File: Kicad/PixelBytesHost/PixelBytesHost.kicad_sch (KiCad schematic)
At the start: 27 parts, among them IC1 2536030320001, J1 TC2030-MCP-NL, Q1 SMMBT5551LT1G, Q2 SMMBT5551LT1G, U1 Pixel Bytes Display, U2 STM32F103CBTx, Y1 CX2520DB12000D0GPSC1

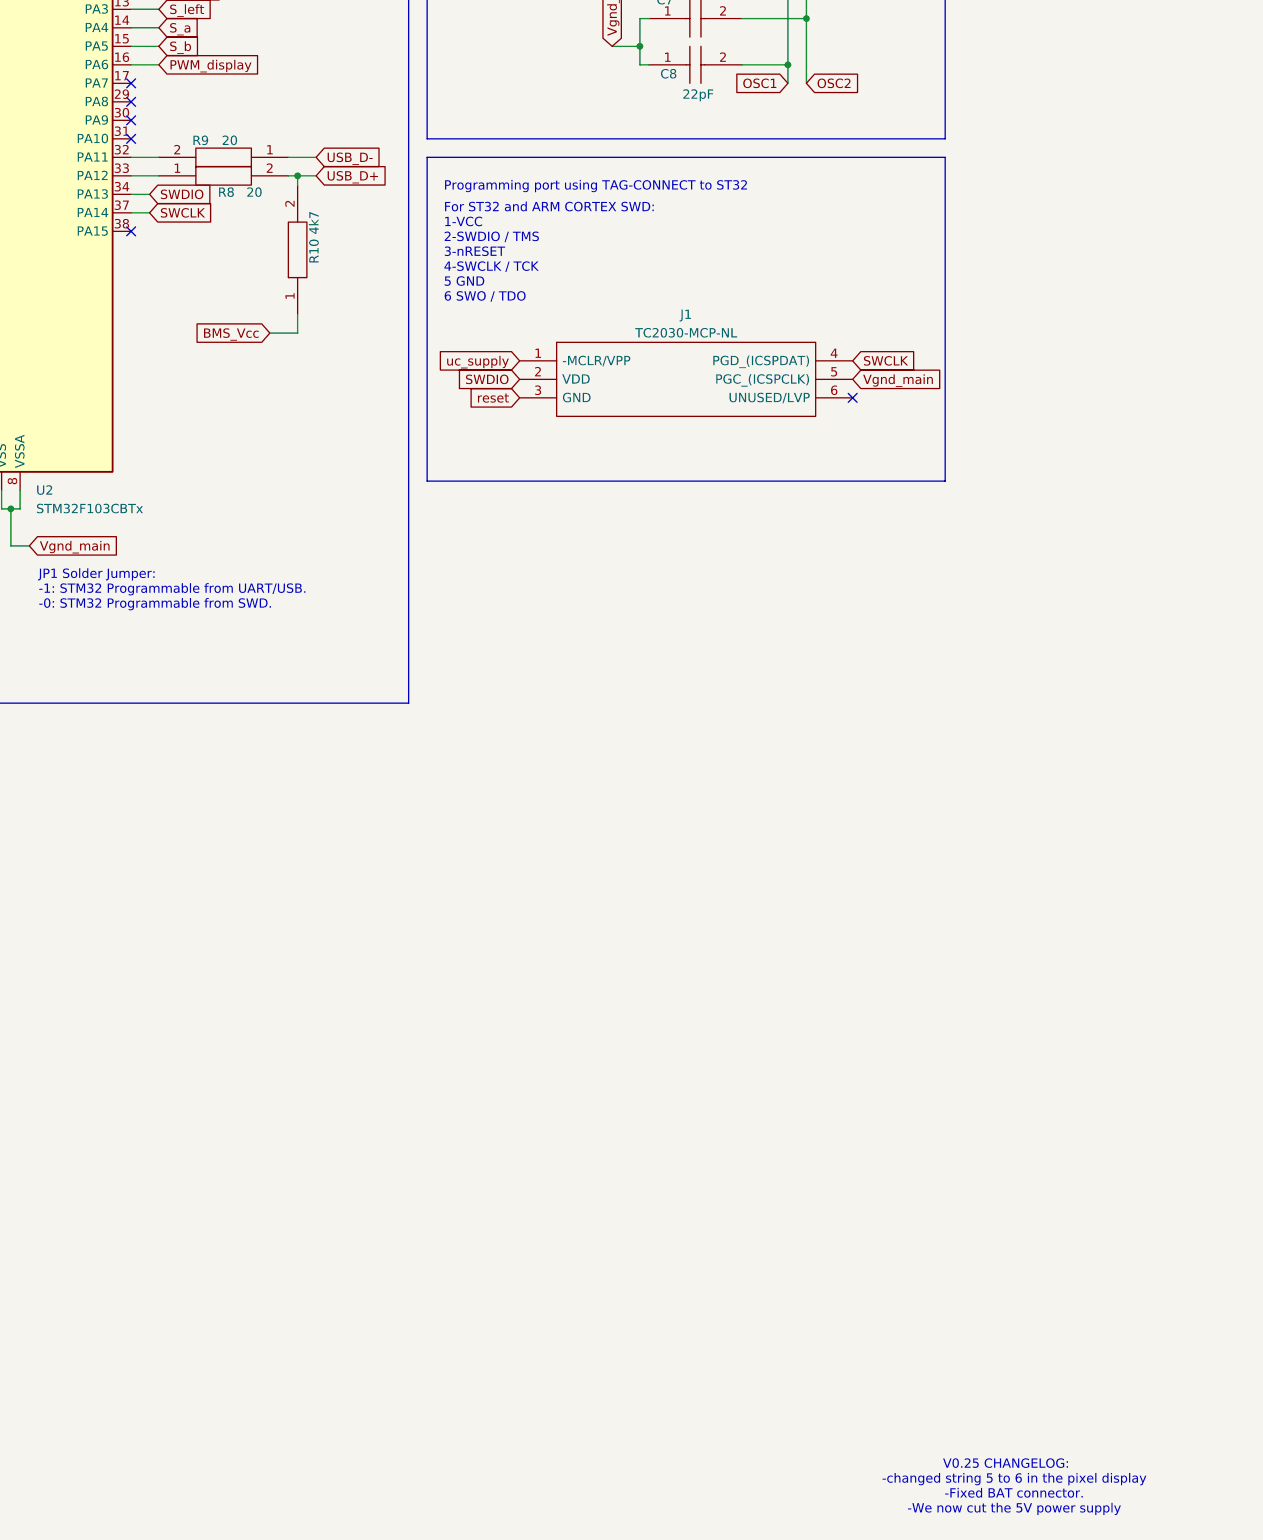
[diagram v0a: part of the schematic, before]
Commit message: Subimos todos los archivos de la v0.25
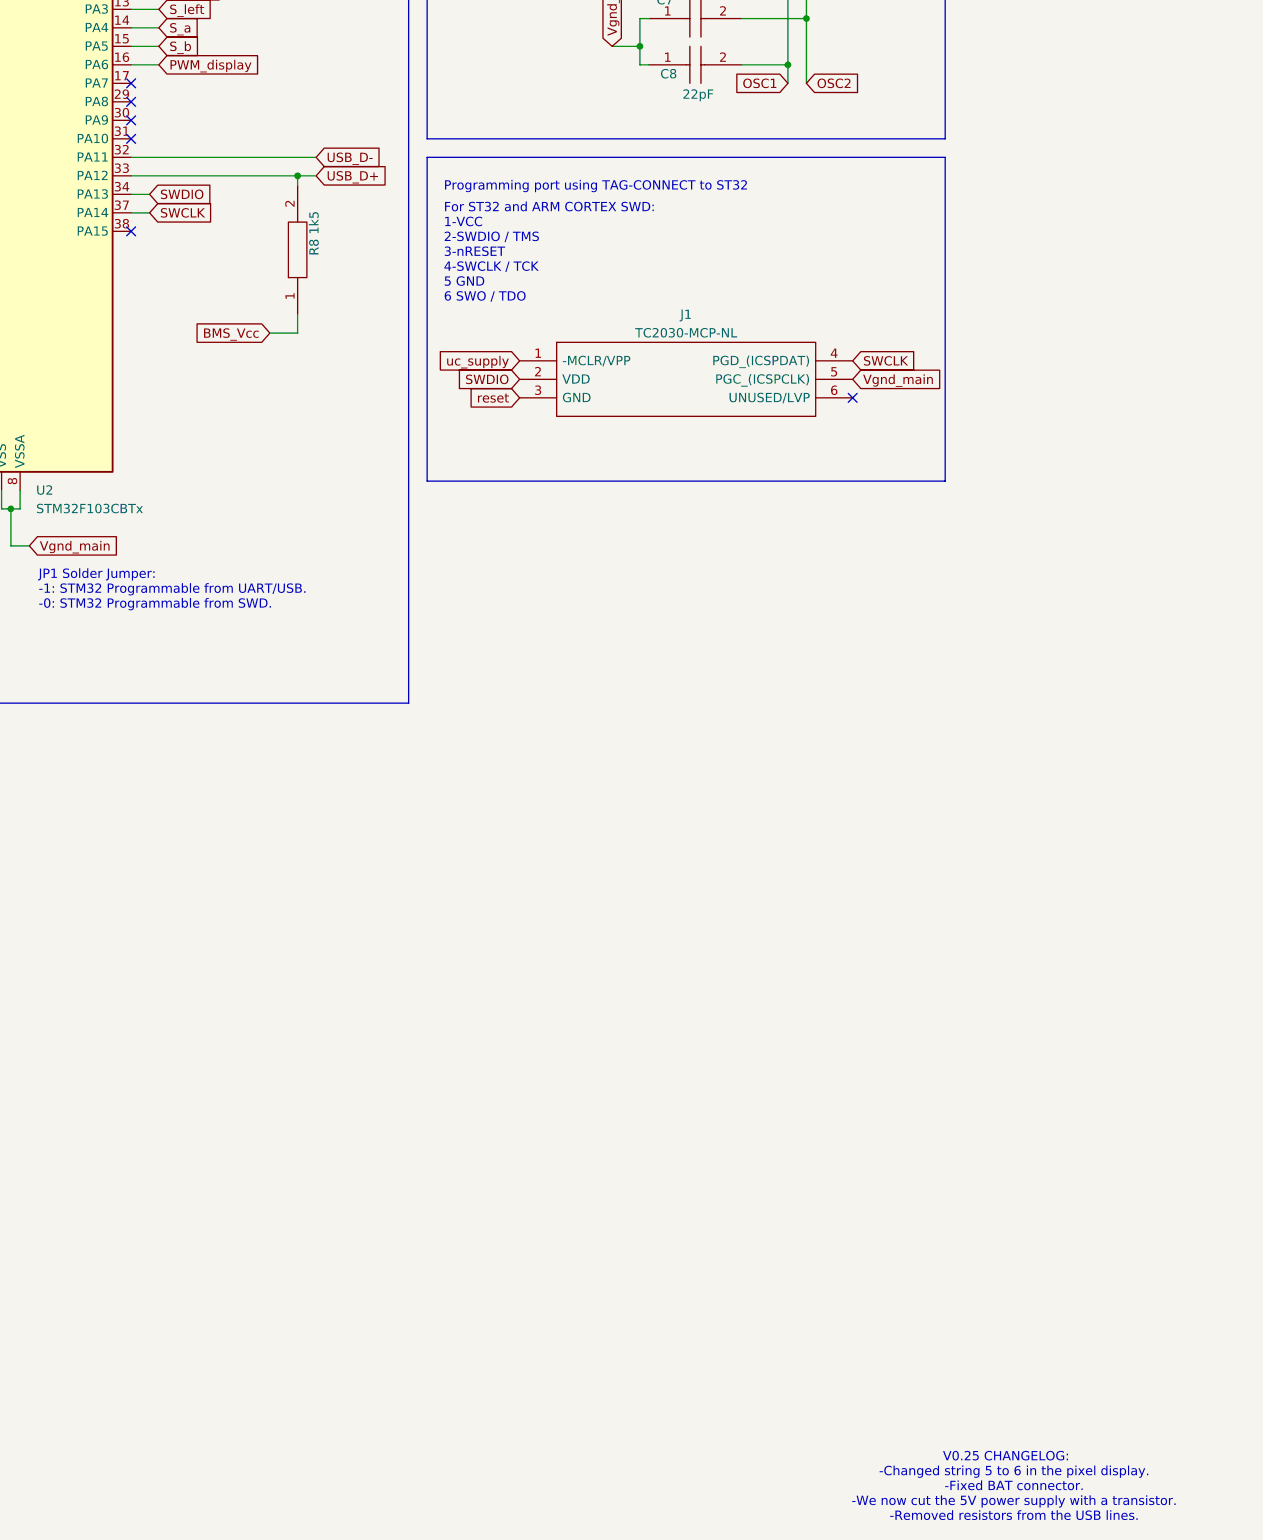
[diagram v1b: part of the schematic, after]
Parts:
- removed R8, R9: 20, Resistor_SMD:R_0805_2012Metric, symbol OpenReflowPlate-rescue:ERJP6WF1303V-Library_Loader
- R8: renamed from R10; value 4k7 -> 1k5
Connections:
- net USB_D+: now also U2.33 (PA12)
- net USB_D-: now also U2.32 (PA11)
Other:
- note added: "V0.25 CHANGELOG: -Changed string 5 to 6 in the pixel display. -Fixed BAT connector. -We now cut the 5V power supply with a transistor. -Removed resistors from the USB lines."
- note removed: "V0.25 CHANGELOG: -changed string 5 to 6 in the pixel display -Fixed BAT connector. -We now cut the 5V power supply"

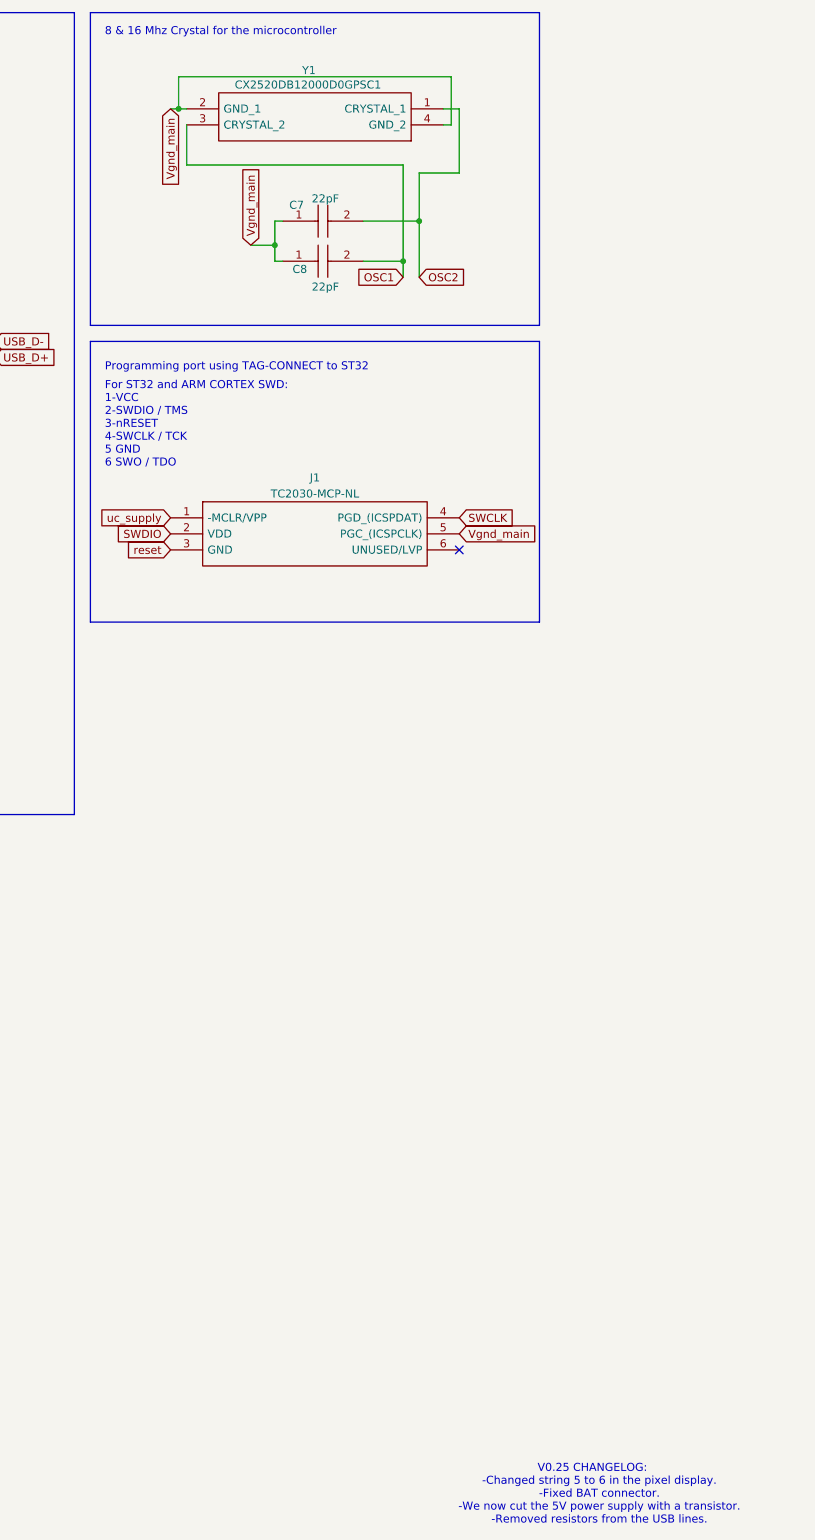
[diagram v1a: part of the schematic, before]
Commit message: Host HW 1.0 finished
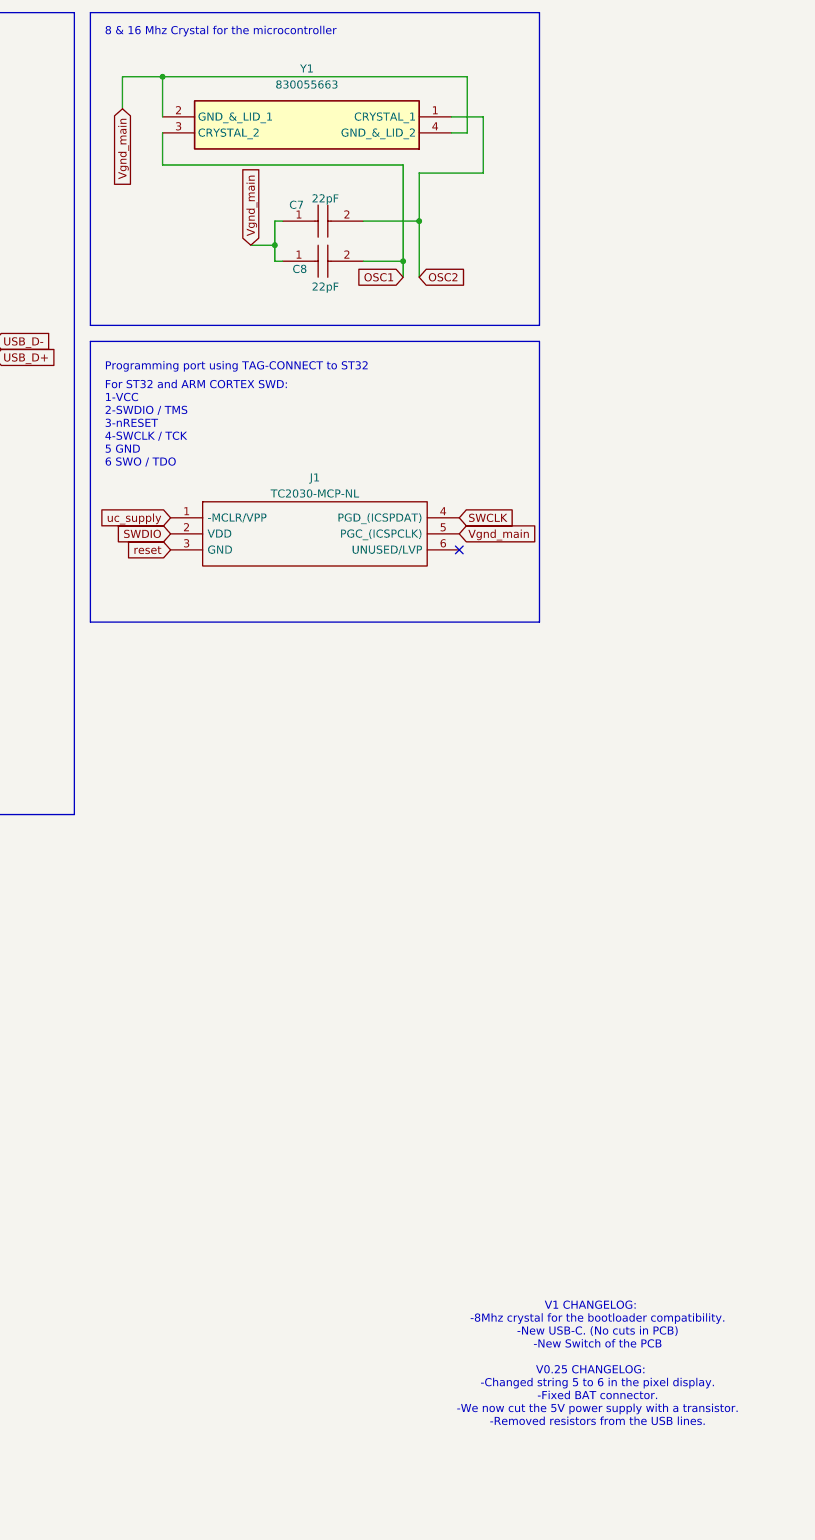
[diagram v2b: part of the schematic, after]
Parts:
- removed Y1: CX2520DB12000D0GPSC1, CX2520DB12000D0GPSC1, symbol User_lib:CX2520DB12000D0GPSC1
- added Y1: 830055663, 830055663, symbol User:830055663
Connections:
- net OSC1: now also Y1.3 (CRYSTAL_2)
- net OSC2: now also Y1.1 (CRYSTAL_1)
- net Vgnd_main: now also Y1.2 (GND_&_LID_1), Y1.4 (GND_&_LID_2)
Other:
- note added: "V1 CHANGELOG: -8Mhz crystal for the bootloader compatibility. -New USB-C. (No cuts in PCB) -New Switch of the PCB V0.25 CHANGELOG: -Changed string 5 to 6 in the pixel display. -Fixed BAT connector. -We now cut the 5V power supply with a transistor. -Removed resistors from the USB lines."
- note removed: "V0.25 CHANGELOG: -Changed string 5 to 6 in the pixel display. -Fixed BAT connector. -We now cut the 5V power supply with a transistor. -Removed resistors from the USB lines."
